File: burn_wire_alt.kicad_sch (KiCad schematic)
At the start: 15 parts, among them J1 Conn_01x02_Pin, J2 Conn_01x02_Pin, U1 ADP2303ARDZ

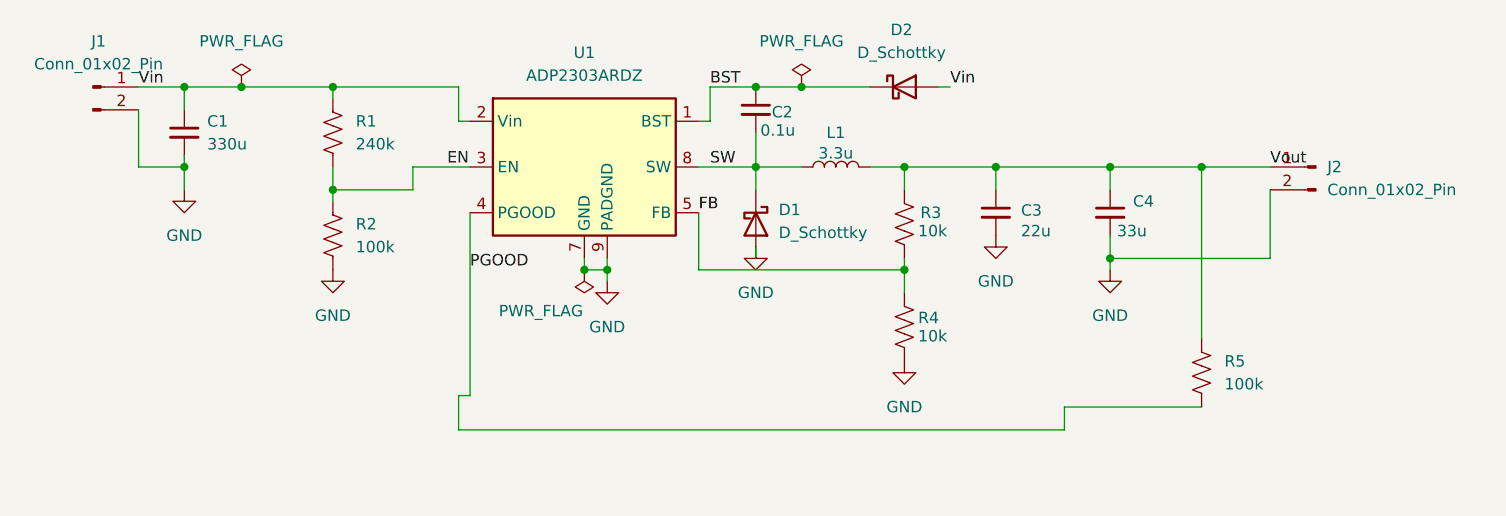
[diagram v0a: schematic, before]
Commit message: new
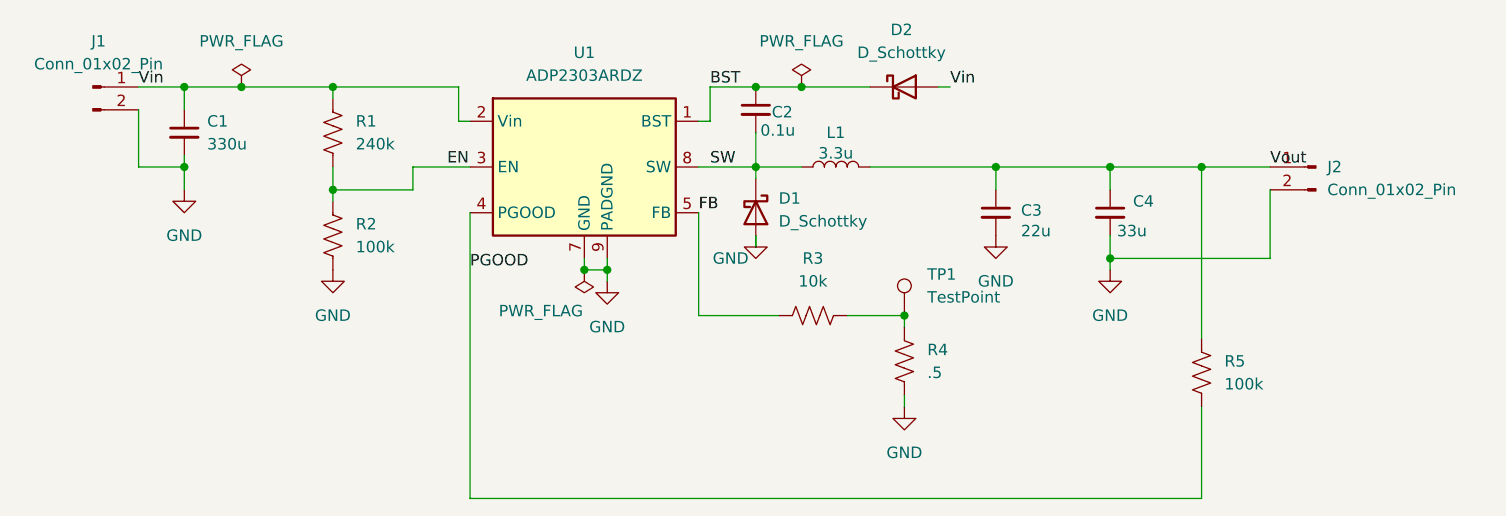
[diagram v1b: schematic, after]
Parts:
- added TP1: TestPoint, Connector_PinSocket_2.54mm:PinSocket_1x01_P2.54mm_Vertical, symbol Connector:TestPoint
- R4: value 10k -> .5; footprint Resistor_SMD:R_0603_1608Metric -> Resistor_SMD:R_2512_6332Metric
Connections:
- net FB: now also R3.1; no longer R3.2, R4.1
- net Vout: no longer R3.1
- new net: R3.2, R4.1, TP1.1
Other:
- moved on the sheet: D1
